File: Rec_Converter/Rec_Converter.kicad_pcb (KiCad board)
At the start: 2 copper layers, 37.8 x 33 mm, 6 parts, among them J1 RJ45, J2 RJ45

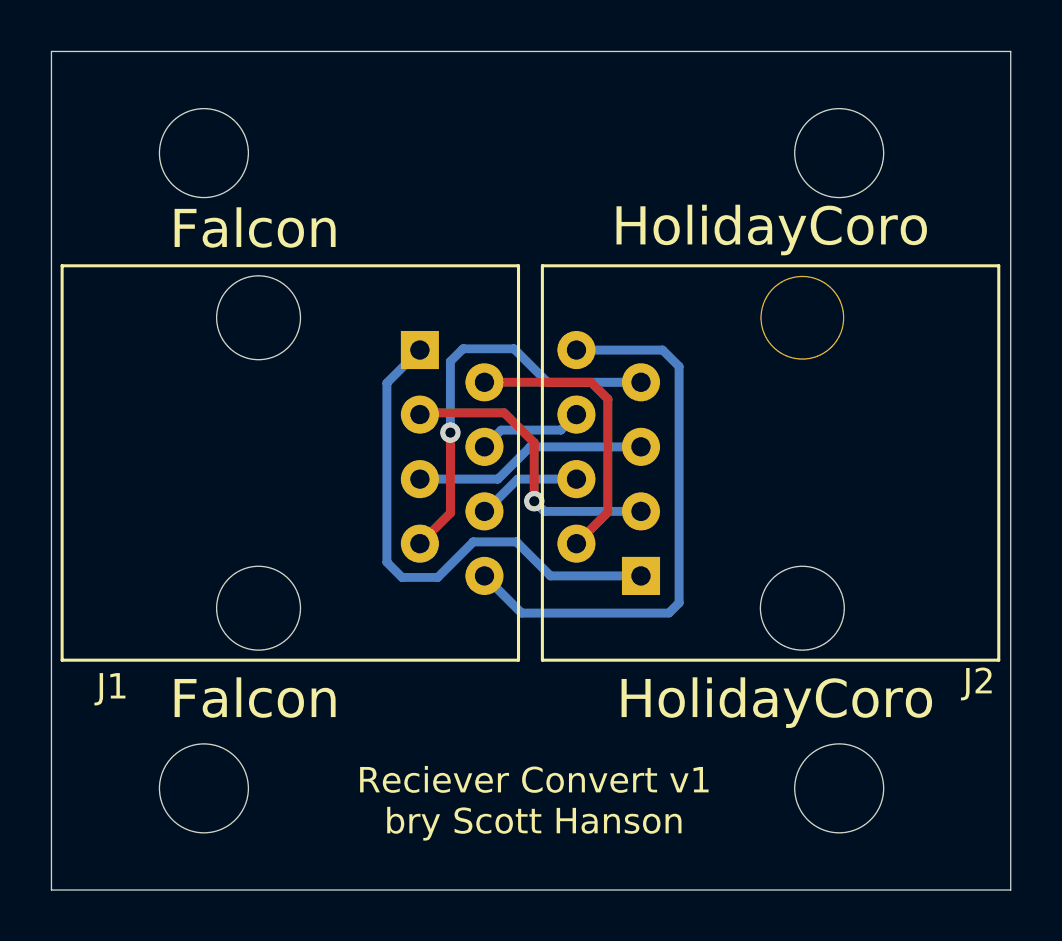
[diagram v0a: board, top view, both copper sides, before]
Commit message: added schematic
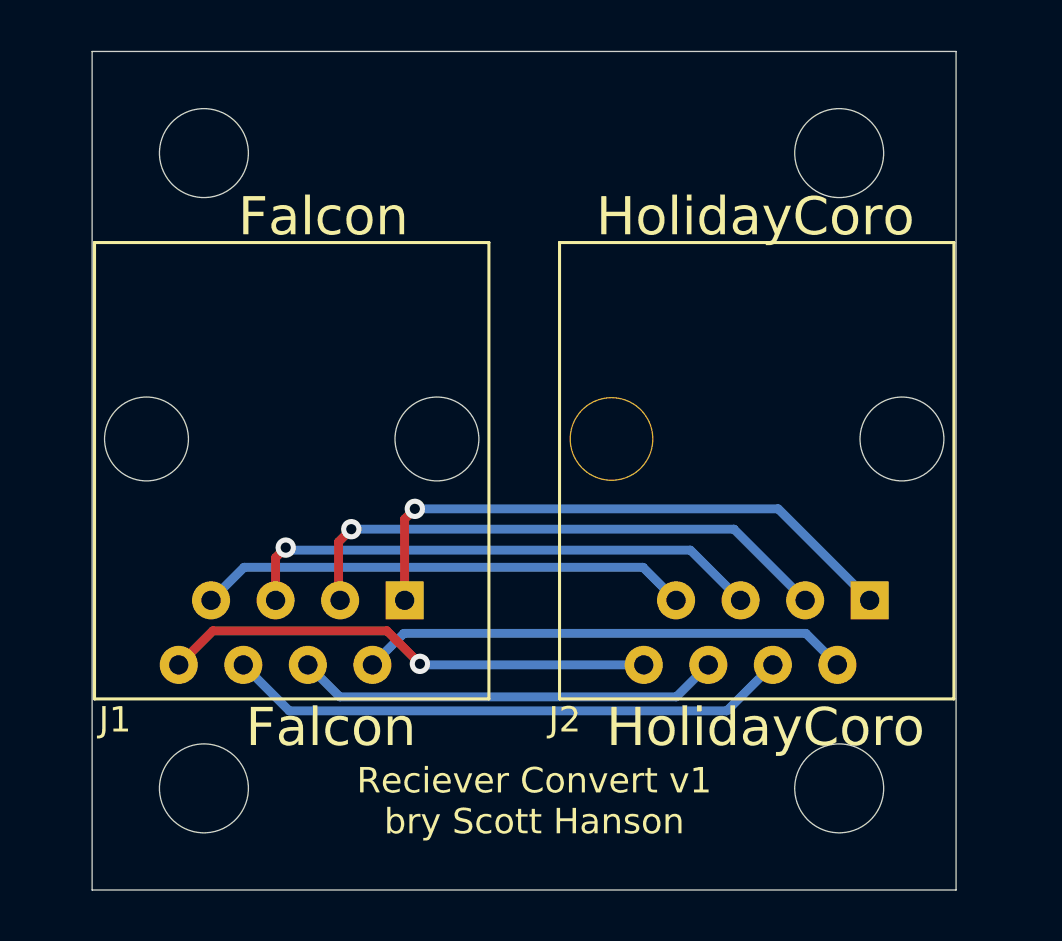
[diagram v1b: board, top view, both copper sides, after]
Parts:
- moved J1 9.87 mm to (146.9, 115.6), turned to 180 degrees
- moved J2 9.05 mm to (165.2, 115.6), turned to 180 degrees
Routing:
- net Net-(J1-Pad6): track 4.15 -> 22.3 mm
- net Net-(J1-Pad4): track 4.15 -> 16.8 mm
- net Net-(J1-Pad5): track 9.23 -> 21.2 mm, vias 0 -> 1
- net Net-(J1-Pad3): track 11.7 -> 22.1 mm
- net Net-(J1-Pad2): track 11.3 -> 19.3 mm
- net Net-(J1-Pad7): track 16.0 -> 19.4 mm, vias 1 -> 0
- net Net-(J1-Pad1): track 20.3 -> 23.2 mm, vias 0 -> 1
- net Net-(J1-Pad8): track 22.0 -> 19.4 mm, vias 0 -> 1
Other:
- board size 37.8 x 33 mm -> 34 x 33 mm
